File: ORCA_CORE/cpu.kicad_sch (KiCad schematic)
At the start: 41 parts, among them J10 Raspberry_Pi_2_3, J11 I2C, J12 I2C, J13 6Vout, J14 5Vout, J15 Conn_01x05_Pin, J16 Conn_01x05_Pin, J20 5Vout, P1 USB_C_Plug_USB2.0, Q6 BSS138, Q7 BSS138, U13 FT230XS, U14 BNO055, U15 NJM78055DL1

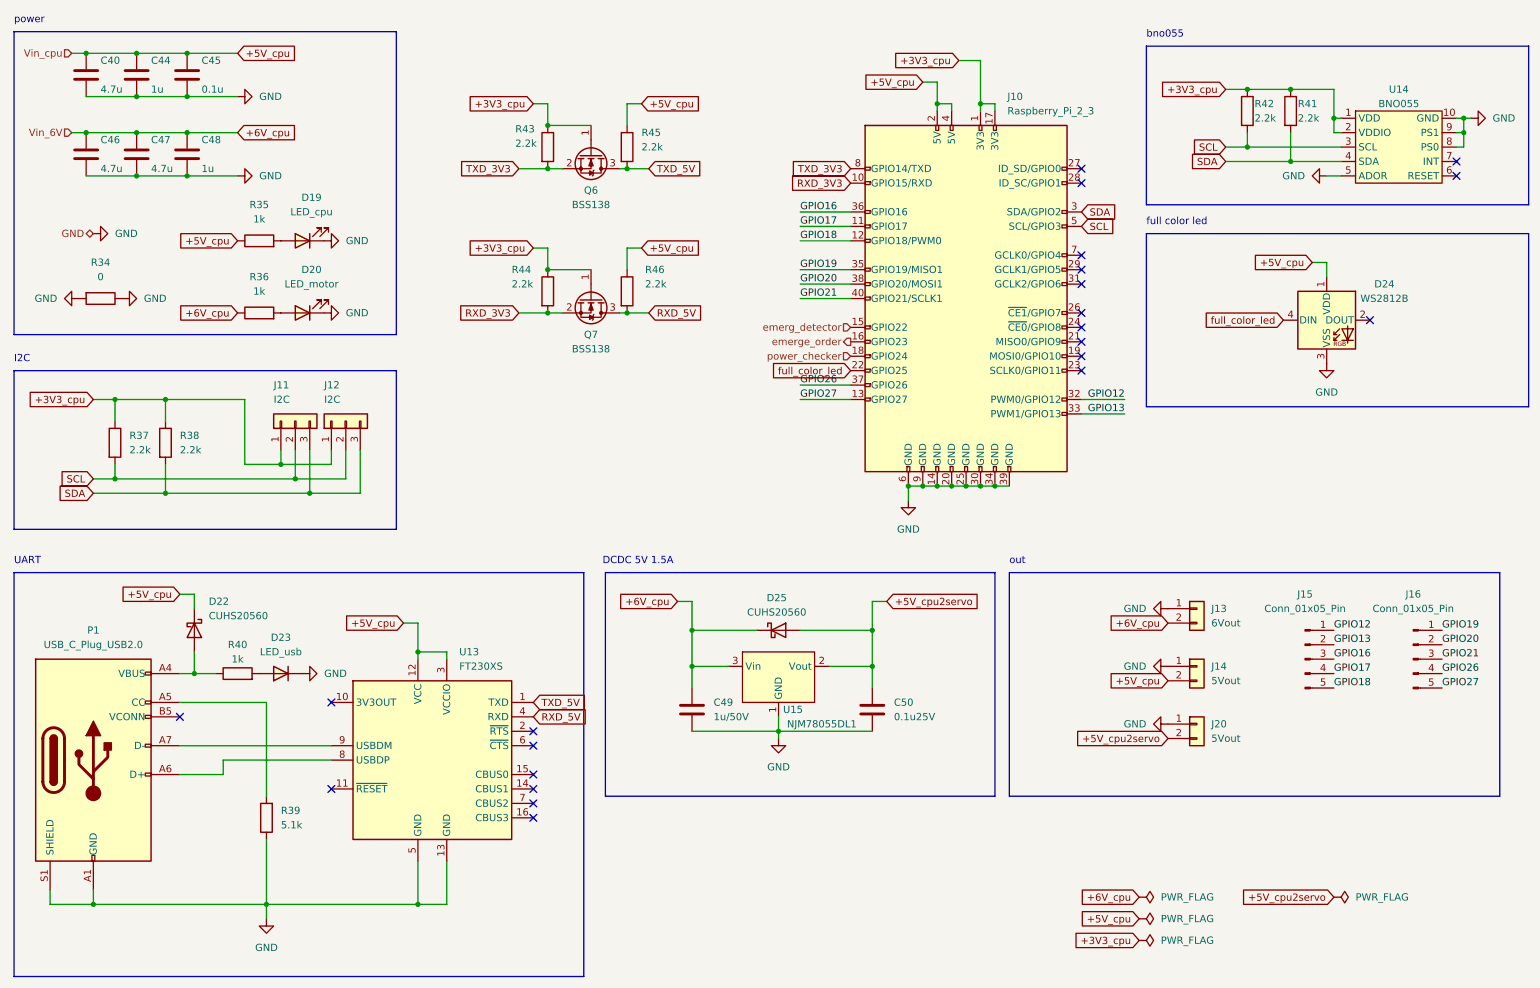
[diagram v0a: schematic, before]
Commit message: attach all the footprints
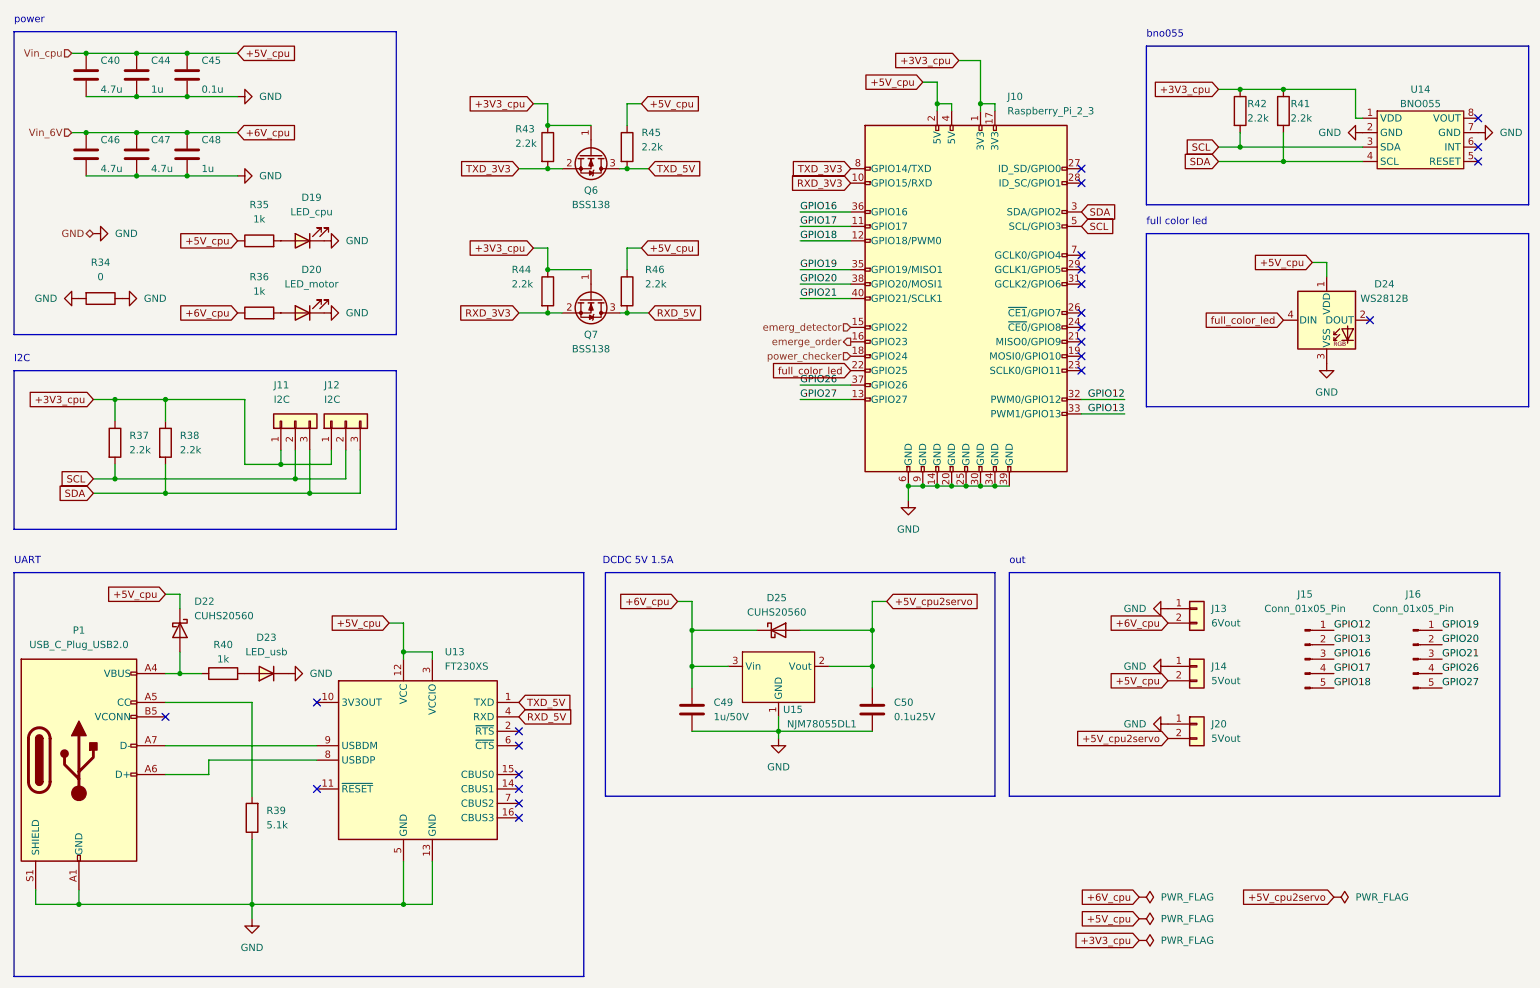
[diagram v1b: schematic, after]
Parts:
- R36: footprint Resistor_SMD:R_0603_1608Metric_Pad0.98x0.95mm_HandSolder -> Relay_THT:RH1-U
- U14: footprint (none) -> IMU:BNO055
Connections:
- net +3V3_cpu: no longer U14.2 (VDDIO)
- net GND: now also U14.2 (GND), U14.7 (GND); no longer U14.10 (GND), U14.5 (ADOR), U14.8 (PS0), U14.9 (PS1)
- no-connect marks 22 -> 23
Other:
- moved on the sheet: D22, D23, P1, R39, R40, R41, R42, U13
